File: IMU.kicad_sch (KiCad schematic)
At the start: 1 part, among them U1 RASPBERRY_PI_ZERO_2_W

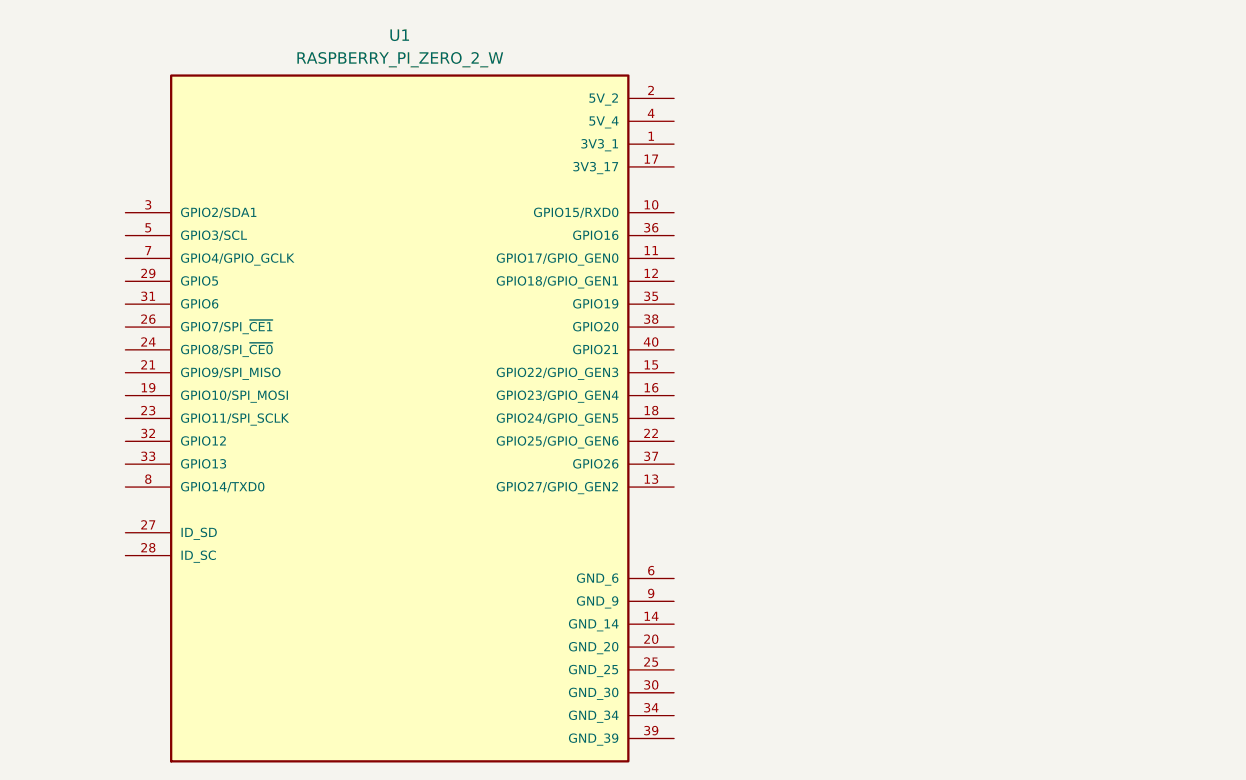
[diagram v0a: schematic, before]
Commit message: IMU schematic made
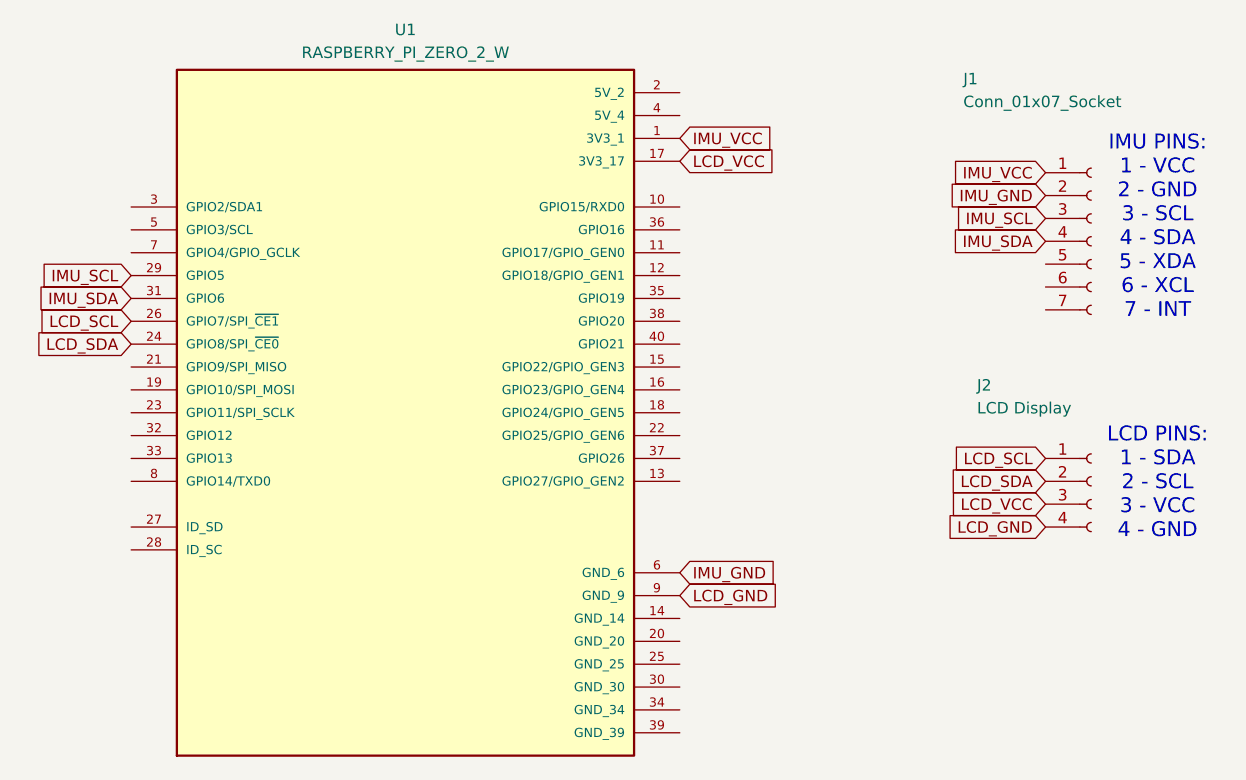
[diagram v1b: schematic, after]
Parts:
- added J1: Conn_01x07_Socket, symbol Connector:Conn_01x07_Socket
- added J2: LCD Display, symbol Connector:Conn_01x04_Socket
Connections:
- net IMU_VCC: now reaches U1.1 (3V3_1)
- net IMU_VCC: now also J1.1 (Pin_1)
- net LCD_VCC: now reaches U1.17 (3V3_17)
- net LCD_VCC: now also J2.3 (Pin_3)
- net LCD_SDA: now reaches U1.24 (GPIO8/SPI_~{CE0})
- net LCD_SDA: now also J2.2 (Pin_2)
- net LCD_SCL: now reaches U1.26 (GPIO7/SPI_~{CE1})
- net LCD_SCL: now also J2.1 (Pin_1)
- net IMU_SCL: now reaches U1.29 (GPIO5)
- net IMU_SCL: now also J1.3 (Pin_3)
- net IMU_SDA: now reaches U1.31 (GPIO6)
- net IMU_SDA: now also J1.4 (Pin_4)
- net IMU_GND: now reaches U1.6 (GND_6)
- net IMU_GND: now also J1.2 (Pin_2)
- net LCD_GND: now reaches U1.9 (GND_9)
- net LCD_GND: now also J2.4 (Pin_4)
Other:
- note added: "IMU PINS: 1 - VCC 2 - GND 3 - SCL 4 - SDA 5 - XDA 6 - XCL 7 - INT"
- note added: "LCD PINS: 1 - SDA 2 - SCL 3 - VCC 4 - GND"
- moved on the sheet: U1
